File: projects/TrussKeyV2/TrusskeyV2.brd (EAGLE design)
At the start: 39.6 x 19 mm, 43 parts, among them J1 M20-9980346, J2 XF2L-0535-1, J3 10104111-0001LF, Q1 ABM-16MHZ, SW1 LS12T2-T, SW2 EVQ11U09K, SW3 ESE31L11T, U2 TPS62200, U3 LC709203, U5 MCP73831T-2ACI/OT, X1 CON-1PIN, X3 CON-1PIN

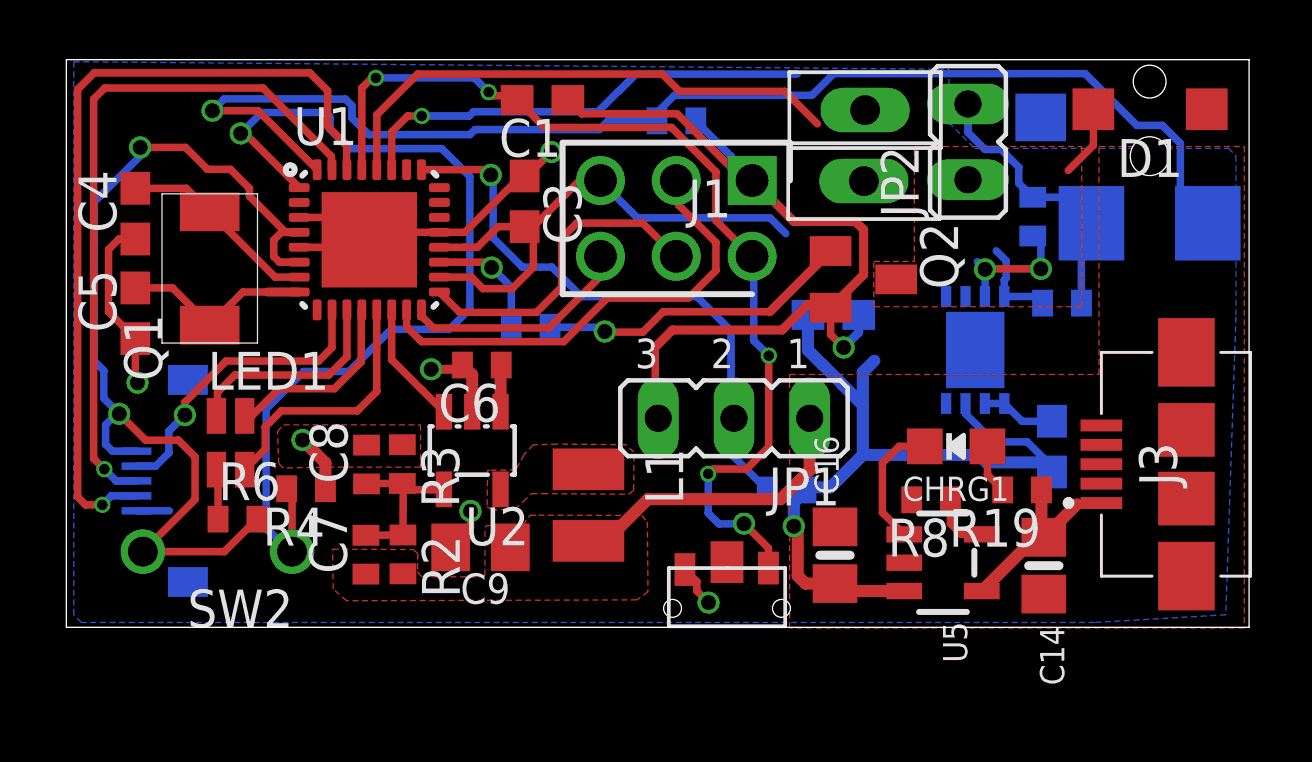
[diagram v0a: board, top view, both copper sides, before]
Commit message: TrussKey v2
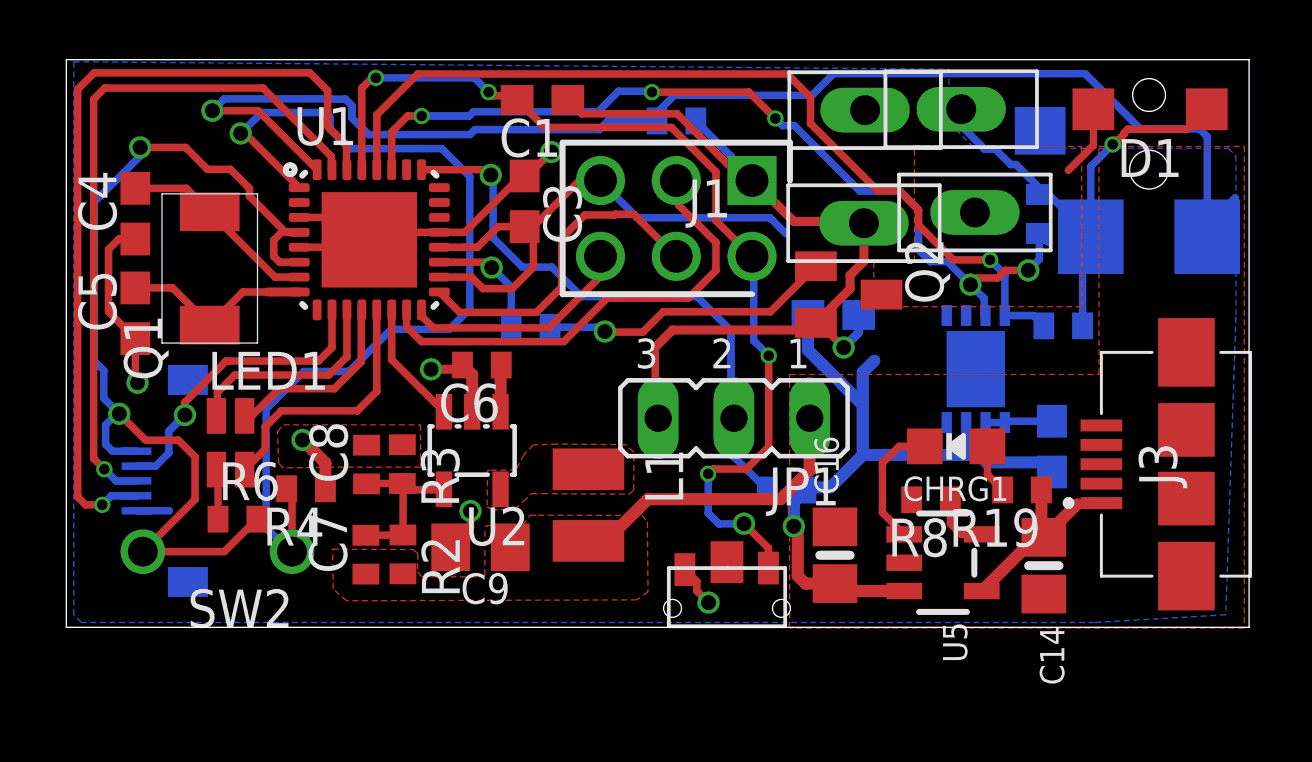
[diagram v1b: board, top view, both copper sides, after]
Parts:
- removed JP2: Solenoid, jumper:JP1
- added X2, X4: CON-1PIN, NewPart:CON-1PIN
- moved X3 1.41 mm to (26.7, 13.5)
- moved R15 0.76 mm to (33.4, 10.1)
- moved Q2 0.71 mm to (26.2, 11.1)
- moved U3 0.64 mm to (30.5, 8.92)
- moved SW3 0.45 mm to (36.3, 15.3)
- moved R16 0.24 mm to (32.6, 13.8)
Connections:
- net N$9: now also X4.P$1; no longer JP2.1
- net VCC: now also X2.P$1; no longer JP2.2
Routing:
- net SDA: track 20.0 -> 29.9 mm, vias 3 -> 5
- net SCL: track 20.9 -> 30.0 mm, vias 0 -> 1
- net VCC: track 88.1 -> 92.5 mm, vias 3 -> 4
- net DETSW: track 42.7 -> 45.5 mm
- net N$10: track 10.6 -> 9.89 mm
